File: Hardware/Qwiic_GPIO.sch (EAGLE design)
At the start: 31 parts, among them J2 SMD, J3 PTH, J4 SMD, U3 TCA9534U

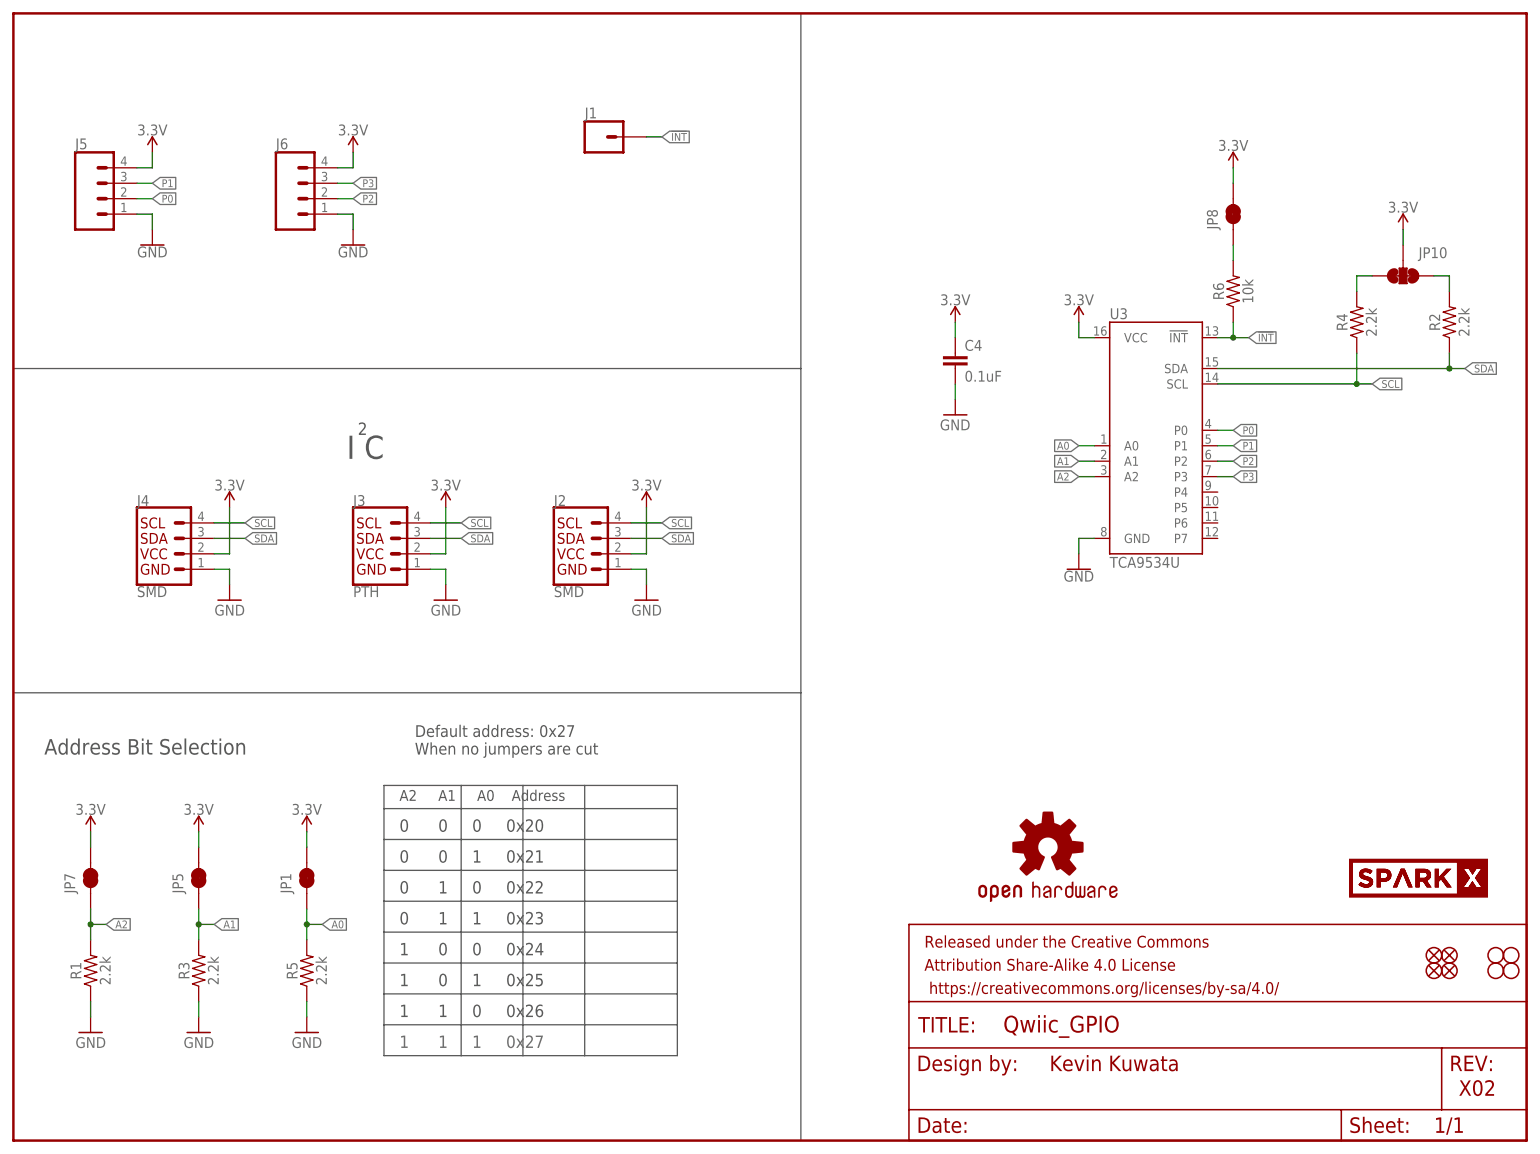
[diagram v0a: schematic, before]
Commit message: Silkscreen
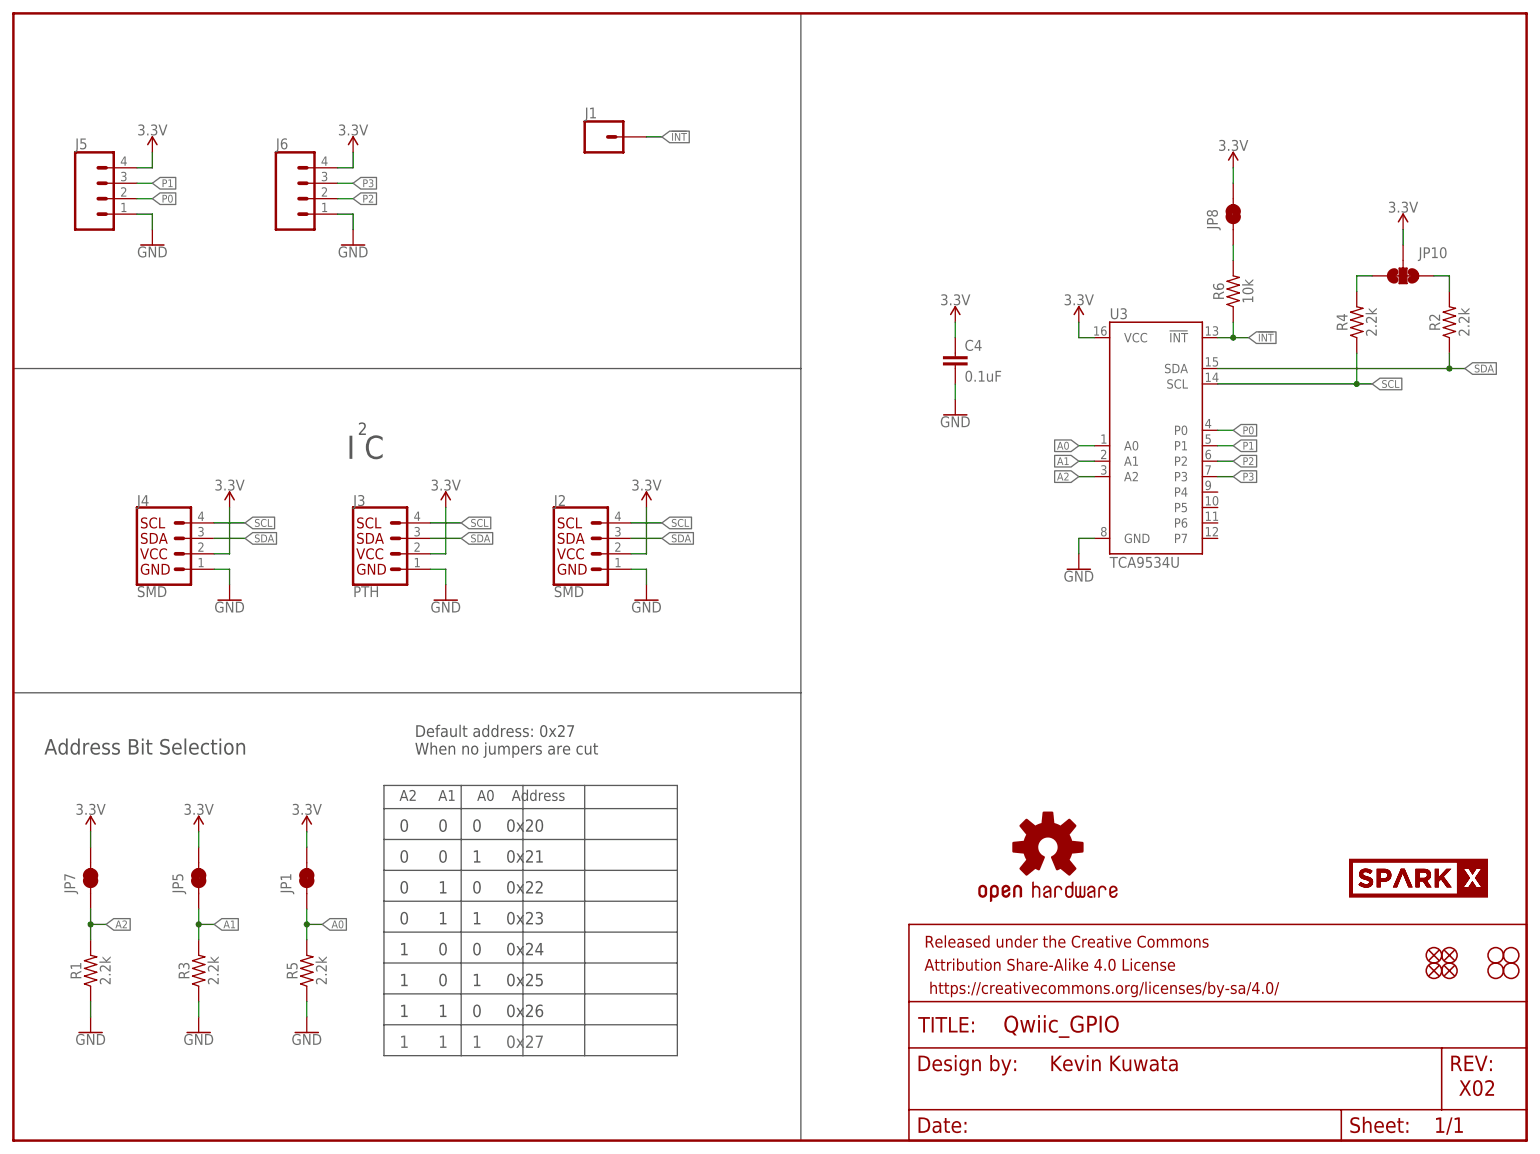
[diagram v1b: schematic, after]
